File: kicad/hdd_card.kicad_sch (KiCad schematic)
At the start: 19 parts, among them J1 POISK, J2 ICSP, J3 SDCARD, J4 UART, U1 28C256, U2 74LS245, U3 28C256, U4 PIC18F47Q10-xP, U5 74LS00, U6 74LS32, U7 74LS74

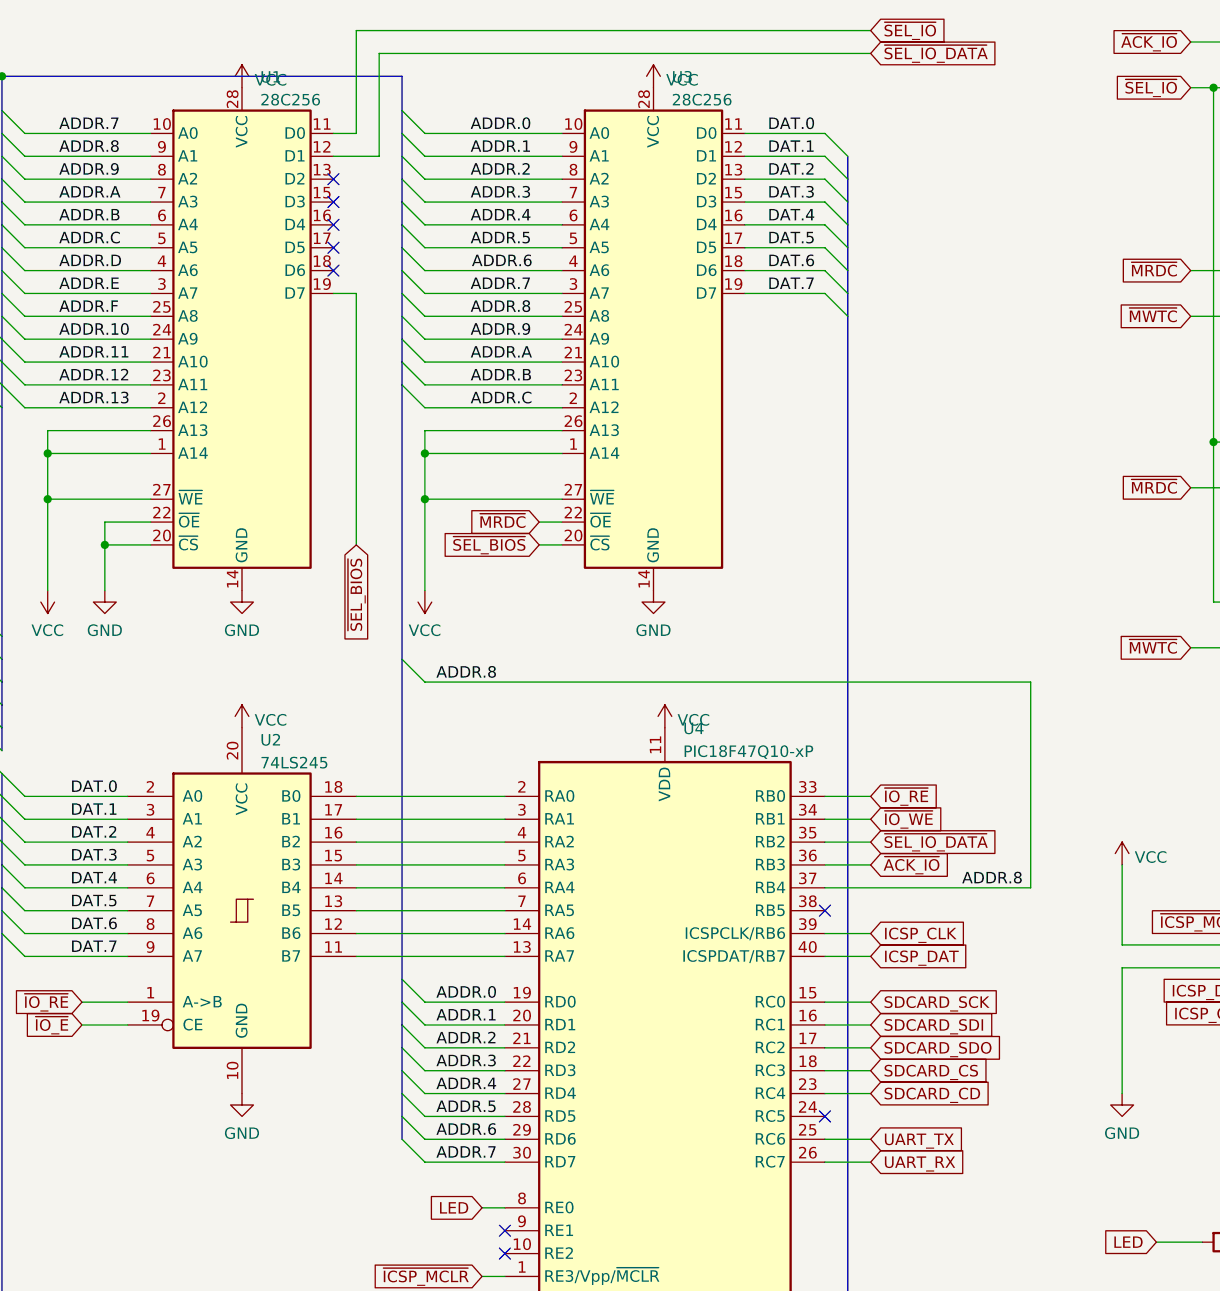
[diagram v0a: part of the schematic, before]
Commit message: 4K IO aperture
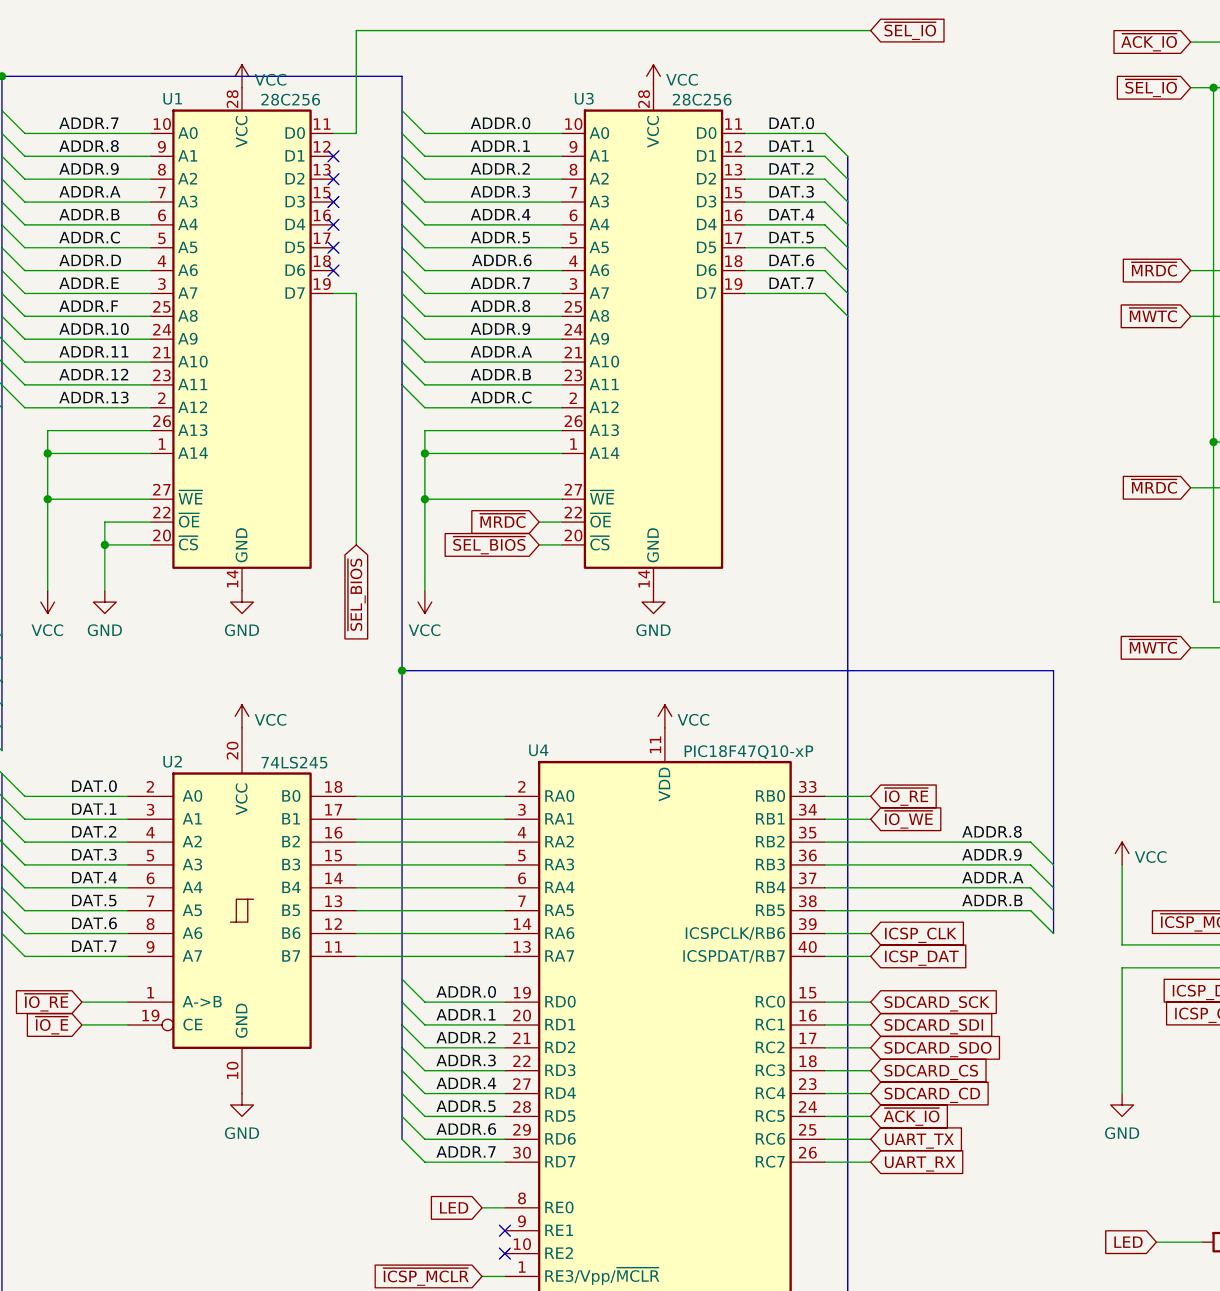
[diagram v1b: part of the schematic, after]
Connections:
- net ADDR.8: now also U4.35 (RB2); no longer U4.37 (RB4)
- net ADDR.9: now also U4.36 (RB3)
- net ADDR.A: now also U4.37 (RB4)
- net ADDR.B: now also U4.38 (RB5)
- net ~{ACK_IO}: now also U4.24 (RC5); no longer U4.36 (RB3)
- net ~{SEL_IO_DATA}: no longer names the net of U1.12 (D1)
- net ~{SEL_IO_DATA}: no longer U4.35 (RB2)
- no-connect marks 38 -> 37
